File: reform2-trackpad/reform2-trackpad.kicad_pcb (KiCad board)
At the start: 2 copper layers, 35 x 40 mm, 24 parts, among them J1 Conn_USB, J2 Conn_01x06_Female, SW6 SW_RST, SW7 SW_HWB, U1 ATmega32U2-AU, U2 TLV75533PDBV, Y1 Crystal_GND24

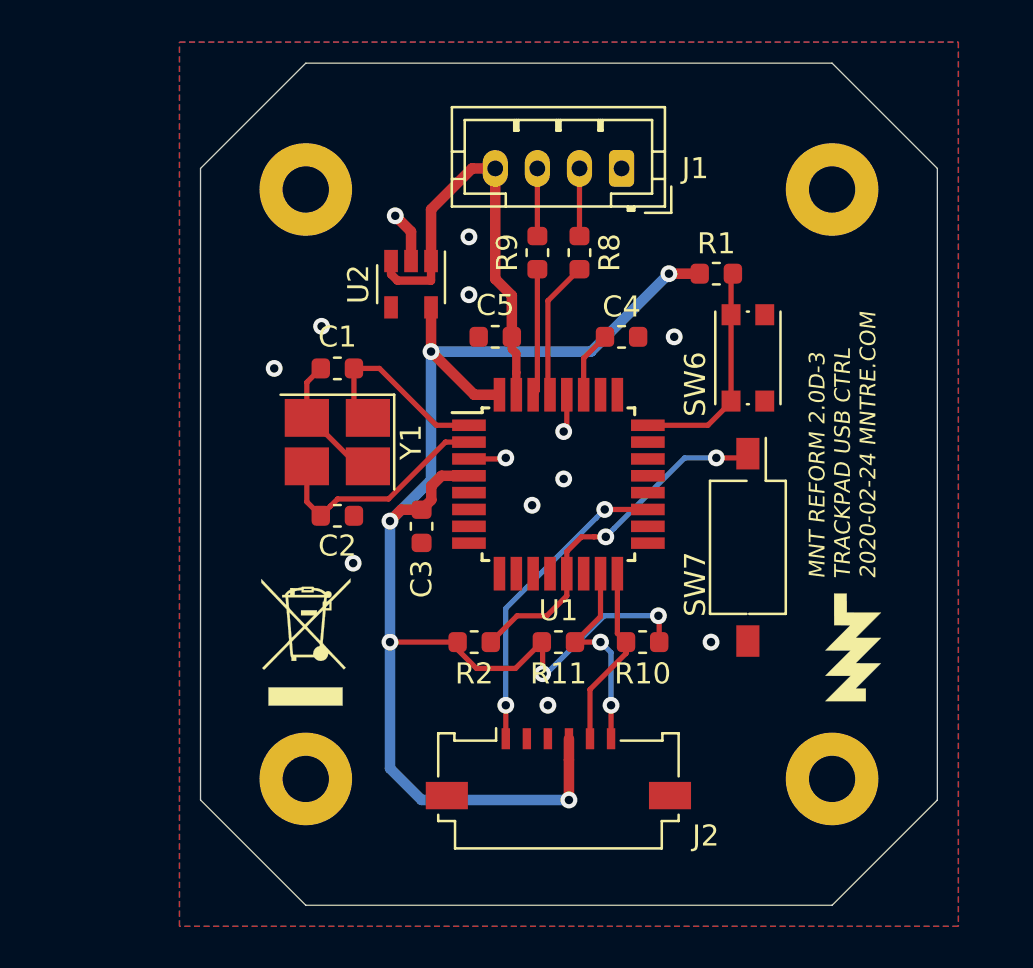
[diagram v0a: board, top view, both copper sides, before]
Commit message: Reform2.0D-3 snapshot of PCBs and input device firmware
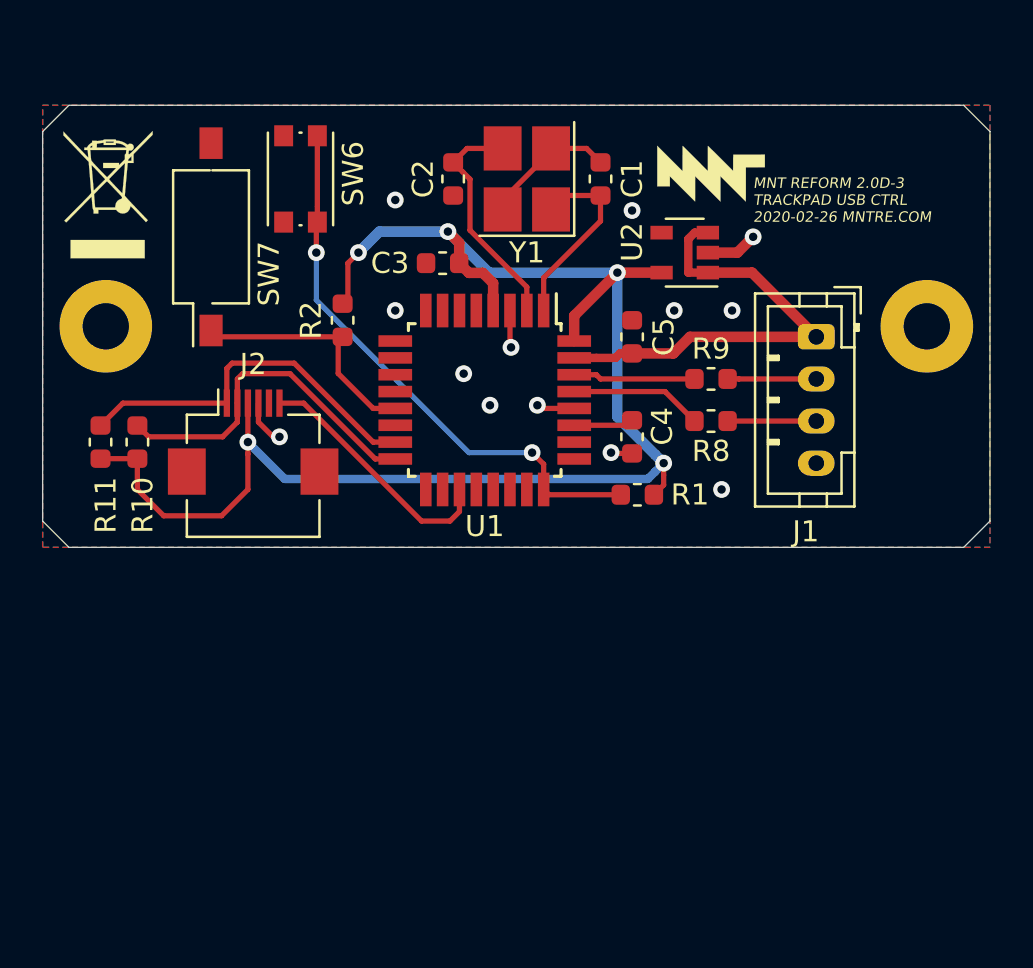
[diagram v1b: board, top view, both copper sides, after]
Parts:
- removed MK7, MK8: Mounting_Hole, MountingHole:MountingHole_2.2mm_M2_Pad
- removed REF**: WEEE-Logo_4.2x6mm_SilkScreen, Symbol:WEEE-Logo_4.2x6mm_SilkScreen
- added MK1: WEEE, Symbol:WEEE-Logo_4.2x6mm_SilkScreen, F.Cu at (176.6, 99.2)
- J2: footprint Connector_FFC-FPC:Molex_200528-0060_1x06-1MP_P1.00mm_Horizontal -> Connector_FFC-FPC:Hirose_FH12-6S-0.5SH_1x06-1MP_P0.50mm_Horizontal
- moved MK6 35.1 mm to (176.5, 105.5), turned to 270 degrees
- moved MK5 30.2 mm to (215.5, 105.5), turned to 270 degrees
- moved SW7 29.5 mm to (181.5, 101.2), turned to 90 degrees
- moved R10 25.8 mm to (178.0, 111.0), turned to 270 degrees
- moved R11 23.7 mm to (176.2, 111.0), turned to 270 degrees
- moved MK13 23.5 mm to (205.2, 98.2), turned to 0 degrees
- moved SW6 22.9 mm to (185.8, 98.5), turned to 90 degrees
- moved J2 20.9 mm to (183.5, 111.0)
- moved C2 16.9 mm to (193.0, 98.5), turned to 90 degrees
- moved R2 16.5 mm to (187.8, 105.2), turned to 90 degrees
- moved C1 15.4 mm to (200.0, 98.5), turned to 90 degrees
- moved Y1 15.4 mm to (196.5, 98.5), turned to 90 degrees
- moved U2 13.1 mm to (204.0, 102.0), turned to 180 degrees
- moved C3 12.5 mm to (192.5, 102.5), turned to 180 degrees
- moved J1 12.2 mm to (210.2, 106.0), turned to 270 degrees
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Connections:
- J1 pad 1: GND -> +5V
- J1 pad 4: +5V -> GND
- J2 pad 1: RDY -> SDA
- J2 pad 2: RST -> SCL
- J2 pad 3: GND -> +3V3
- J2 pad 4: +3V3 -> GND
- J2 pad 5: SCL -> RST
- J2 pad 6: SDA -> RDY
- R8 pad 1: Net-(J1-Pad2) -> Net-(J1-Pad3)
- R9 pad 2: Net-(J1-Pad3) -> Net-(J1-Pad2)
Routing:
- net Net-(R1-Pad2): track 10.5 -> 26.8 mm, vias 0 -> 2
- net SDA: track 9.76 -> 17.7 mm, vias 2 -> 0
- net SCL: track 8.72 -> 16.6 mm
- net Net-(R2-Pad1): track 17.1 -> 11.9 mm, vias 2 -> 0
- net GND: track 12.5 -> 15.7 mm
- net +3V3: track 76.0 -> 73.2 mm, vias 7 -> 5
- net RDY: track 14.9 -> 12.1 mm, vias 2 -> 0
- net Net-(J1-Pad3): track 3.21 -> 4.21 mm
- net Net-(J1-Pad2): track 3.21 -> 4.21 mm
- net +5V: track 21.1 -> 21.9 mm
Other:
- board size 35 x 40 mm -> 45 x 21 mm
- board text added: "MNT REFORM 2.0D-3 TRACKPAD USB CTRL 2020-02-26 MNTRE.COM"
- board text removed: "MNT REFORM 2.0D-3 TRACKPAD USB CTRL 2020-02-24 MNTRE.COM"
